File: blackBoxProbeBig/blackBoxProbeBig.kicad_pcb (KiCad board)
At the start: 4 copper layers, 44 x 44 mm, 84 parts, among them J1 USB-ID, J2 JTAG_2X05, J3 JTAG_2X05, J4 Conn_01x04, Q1 Q_NMOS_DUAL, Q2 Q_PMOS_DUAL, U1 MCP1702-MB, U2 USBLC6-2, U3 STM32F103CBT, U4 74X2T45, U5 74X2T45, U6 74X2T45, U7 74X2T45, Y1 8.000MHz

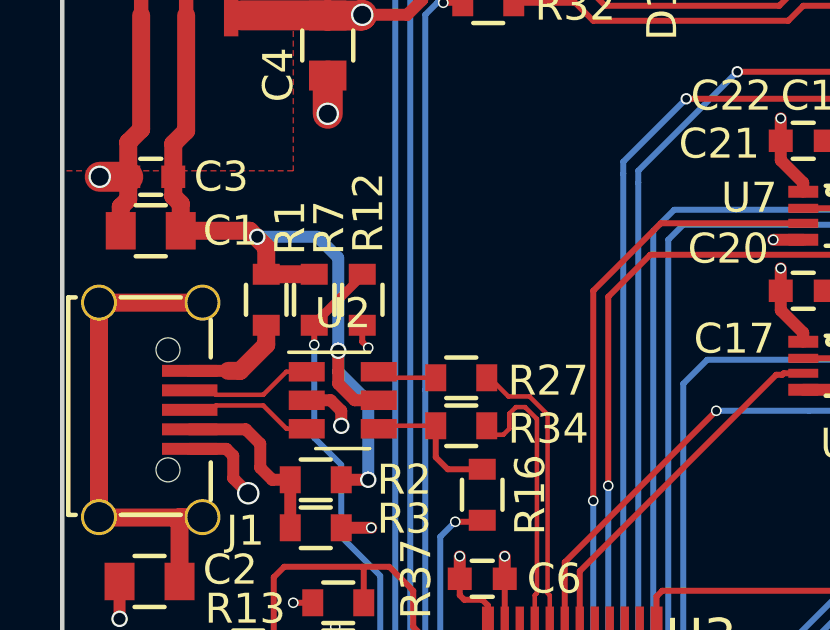
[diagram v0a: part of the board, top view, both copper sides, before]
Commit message: small updates
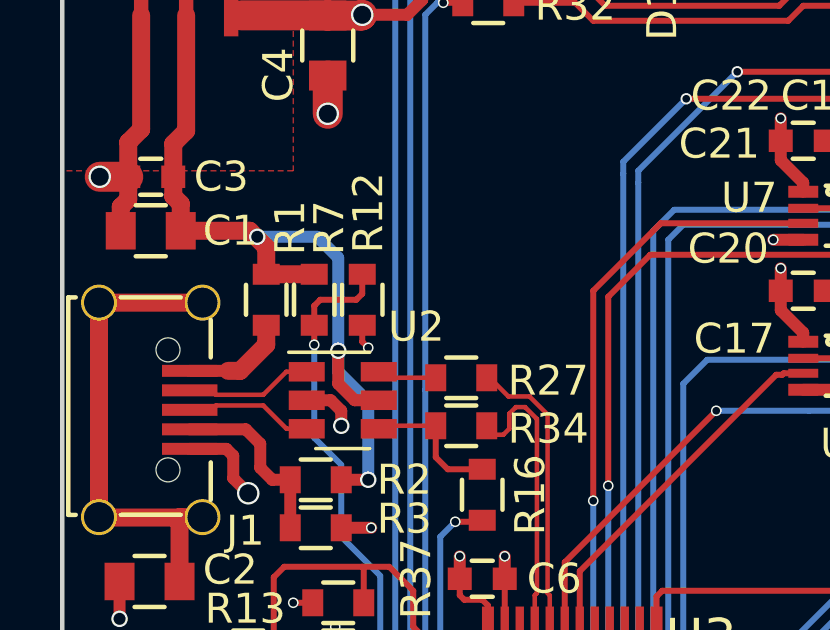
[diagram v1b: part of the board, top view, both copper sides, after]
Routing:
- net /USB_V: track 29.0 -> 29.8 mm
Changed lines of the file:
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@@
     (thickness 1.6)
     (drawings 10)
-    (tracks 780)
+    (tracks 784)
     (zones 0)
     (modules 84)
@@
   )
   (setup
-    (last_trace_width 0.127)
+    (last_trace_width 0.2)
     (user_trace_width 0.1524)
     (user_trace_width 0.2)
@@
     (tags SOT-23-6)
     (attr smd)
-    (fp_text reference U2 (at 0 -2.9) (layer F.SilkS)
+    (fp_text reference U2 (at 2.45 -2.45) (layer F.SilkS)
       (effects (font (size 1 1) (thickness 0.15)))
     )
@@
   (via (at 22.7 168.8) (size 0.3556) (drill 0.254) (layers F.Cu B.Cu) (net 36))
   (segment (start 22.7 168.15) (end 22.7 168.7) (width 0.2) (layer F.Cu) (net 36))
-  (segment (start 22.7 168.1) (end 24.3 166.5) (width 0.3) (layer F.Cu) (net 36))
   (segment (start 24.3 166.5) (end 24.3 166.45) (width 0.3) (layer F.Cu) (net 36))
   (segment (start 22.7 168.15) (end 22.7 168.1) (width 0.3) (layer F.Cu) (net 36))
+  (segment (start 22.7 168.15) (end 22.7 167.5) (width 0.2) (layer F.Cu) (net 36))
+  (segment (start 22.7 167.5) (end 22.9 167.3) (width 0.2) (layer F.Cu) (net 36))
+  (segment (start 22.9 167.3) (end 24.1 167.3) (width 0.2) (layer F.Cu) (net 36))
+  (segment (start 24.3 167.1) (end 24.3 166.45) (width 0.2) (layer F.Cu) (net 36))
+  (segment (start 24.1 167.3) (end 24.3 167.1) (width 0.2) (layer F.Cu) (net 36))
   (segment (start 22.81 179.89) (end 22.1 180.6) (width 0.2) (layer F.Cu) (net 37))
   (segment (start 22.1 180.6) (end 21.35 180.6) (width 0.2) (layer F.Cu) (net 37))
